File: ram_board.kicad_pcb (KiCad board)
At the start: 2 copper layers, 28.6 x 73 mm, 6 parts, among them J1 Conn_02x20_Odd_Even, J2 Conn_02x05_Odd_Even, U1 IS61LV5128AL-10TLI, U2 SST39VF040-70-4C-NHE

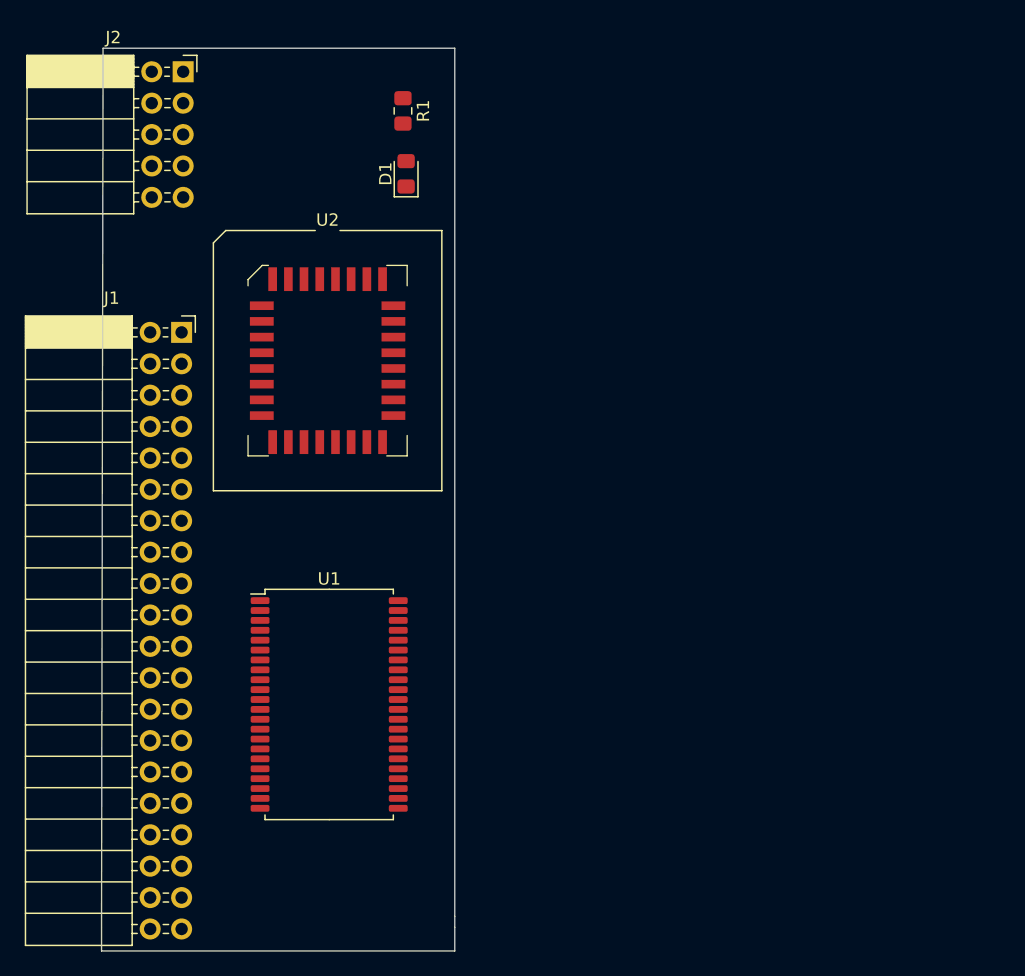
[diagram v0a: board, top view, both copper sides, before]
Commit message: Wiring up
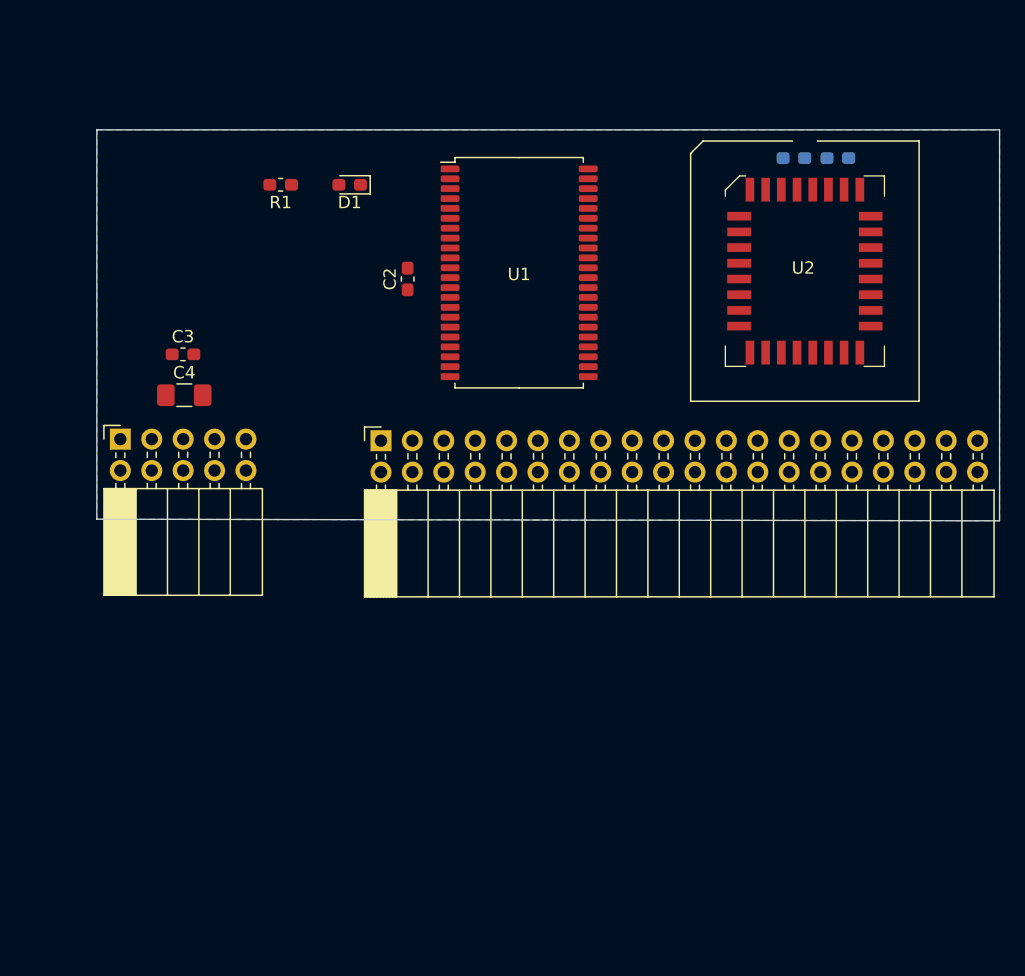
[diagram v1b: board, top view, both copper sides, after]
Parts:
- added C1: 100nF, Capacitor_SMD:C_0603_1608Metric_Pad1.05x0.95mm_HandSolder, B.Cu at (173.5, 74.8)
- added C2: 100nF, Capacitor_SMD:C_0603_1608Metric_Pad1.05x0.95mm_HandSolder, F.Cu at (142.2, 84.6)
- added C3: 100nF, Capacitor_SMD:C_0603_1608Metric_Pad1.05x0.95mm_HandSolder, F.Cu at (124.1, 90.7)
- added C4: 100uF, Capacitor_SMD:C_1206_3216Metric_Pad1.42x1.75mm_HandSolder, F.Cu at (124.2, 94.0)
- added G***: LOGO, Logos:asian_tiger, F.Cu at (160.8, 85.5)
- added R2: 10K, Resistor_SMD:R_0603_1608Metric_Pad1.05x0.95mm_HandSolder, B.Cu at (177.0, 74.8)
- D1: footprint LED_SMD:LED_0805_2012Metric_Pad1.15x1.40mm_HandSolder -> LED_SMD:LED_0603_1608Metric_Pad1.05x0.95mm_HandSolder
- R1: footprint Resistor_SMD:R_0805_2012Metric_Pad1.15x1.40mm_HandSolder -> Resistor_SMD:R_0603_1608Metric_Pad1.05x0.95mm_HandSolder
- moved U2 39.3 mm to (174.4, 83.9)
- moved U1 38.2 mm to (151.3, 84.1)
- moved J2 30.1 mm to (119.0, 97.5), turned to 90 degrees
- moved J1 18.4 mm to (140.1, 97.7), turned to 90 degrees
- moved R1 11.6 mm to (132.0, 77.0), turned to 180 degrees
- moved D1 4.65 mm to (137.6, 77.0), turned to 180 degrees
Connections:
- J1 pad 1: (no net) -> /A0
- J1 pad 10: (no net) -> /A9
- J1 pad 11: (no net) -> /A10
- J1 pad 12: (no net) -> /A11
- J1 pad 13: (no net) -> /A12
- J1 pad 14: (no net) -> /A13
- J1 pad 15: (no net) -> /A14
- J1 pad 16: (no net) -> /A15
- J1 pad 17: (no net) -> /A16
- J1 pad 18: (no net) -> /A17
- J1 pad 19: (no net) -> /A18
- J1 pad 2: (no net) -> /A1
- J1 pad 21: (no net) -> /RAM_CE
- J1 pad 22: (no net) -> /D0
- J1 pad 23: (no net) -> /RAM_OE
- J1 pad 24: (no net) -> /D1
- J1 pad 25: (no net) -> /RAM_WE
- J1 pad 26: (no net) -> /D2
- J1 pad 28: (no net) -> /D3
- J1 pad 3: (no net) -> /A2
- J1 pad 32: (no net) -> GND
- J1 pad 33: (no net) -> GND
- J1 pad 34: (no net) -> /D4
- J1 pad 36: (no net) -> /D5
- J1 pad 38: (no net) -> /D6
- J1 pad 39: (no net) -> GND
- J1 pad 4: (no net) -> /A3
- J1 pad 40: (no net) -> /D7
- J1 pad 5: (no net) -> /A4
- J1 pad 6: (no net) -> /A5
- J1 pad 7: (no net) -> /A6
- J1 pad 8: (no net) -> /A7
- J1 pad 9: (no net) -> /A8
- J2 pad 10: (no net) -> GND
- J2 pad 3: (no net) -> +3V3
- J2 pad 4: (no net) -> +3V3
- J2 pad 7: (no net) -> GND
- J2 pad 8: (no net) -> GND
- J2 pad 9: (no net) -> GND
- R1 pad 2: (no net) -> +3V3
- U1 pad 10: (no net) -> /D1
- U1 pad 11: Net-(U1-Pad11) -> +3V3
- U1 pad 12: Net-(U1-Pad12) -> GND
- U1 pad 13: (no net) -> /D2
- U1 pad 14: (no net) -> /D3
- U1 pad 15: (no net) -> /RAM_WE
- U1 pad 16: (no net) -> /A5
- U1 pad 17: (no net) -> /A6
- U1 pad 18: (no net) -> /A7
- U1 pad 19: (no net) -> /A8
- U1 pad 20: (no net) -> /A9
- U1 pad 26: (no net) -> /A10
- U1 pad 27: (no net) -> /A11
- U1 pad 28: (no net) -> /A12
- U1 pad 29: (no net) -> /A13
- U1 pad 3: (no net) -> /A0
- U1 pad 30: (no net) -> /A14
- U1 pad 31: (no net) -> /D4
- U1 pad 32: (no net) -> /D5
- U1 pad 33: Net-(U1-Pad11) -> +3V3
- U1 pad 34: Net-(U1-Pad12) -> GND
- U1 pad 35: (no net) -> /D6
- U1 pad 36: (no net) -> /D7
- U1 pad 37: (no net) -> /RAM_OE
- U1 pad 38: (no net) -> /A15
- U1 pad 39: (no net) -> /A16
- U1 pad 4: (no net) -> /A1
- U1 pad 40: (no net) -> /A17
- U1 pad 41: (no net) -> /A18
- U1 pad 5: (no net) -> /A2
- U1 pad 6: (no net) -> /A3
- U1 pad 7: (no net) -> /A4
- U1 pad 8: (no net) -> /RAM_CE
- U1 pad 9: (no net) -> /D0
- U2 pad 1: (no net) -> /A18
- U2 pad 10: (no net) -> /A2
- U2 pad 11: (no net) -> /A1
- U2 pad 12: (no net) -> /A0
- U2 pad 13: (no net) -> /D0
- U2 pad 14: (no net) -> /D1
- U2 pad 15: (no net) -> /D2
- U2 pad 17: (no net) -> /D3
- U2 pad 18: (no net) -> /D4
- U2 pad 19: (no net) -> /D5
- U2 pad 2: (no net) -> /A16
- U2 pad 20: (no net) -> /D6
- U2 pad 21: (no net) -> /D7
- U2 pad 22: (no net) -> /RAM_CE
- U2 pad 23: (no net) -> /A10
- U2 pad 24: (no net) -> /RAM_OE
- U2 pad 25: (no net) -> /A11
- U2 pad 26: (no net) -> /A9
- U2 pad 27: (no net) -> /A8
- U2 pad 28: (no net) -> /A13
- U2 pad 29: (no net) -> /A14
- U2 pad 3: (no net) -> /A15
- U2 pad 30: (no net) -> /A17
- U2 pad 31: (no net) -> Net-(R2-Pad1)
- U2 pad 32: (no net) -> +3V3
- U2 pad 4: (no net) -> /A12
- U2 pad 5: (no net) -> /A7
- U2 pad 6: (no net) -> /A6
- U2 pad 7: (no net) -> /A5
- U2 pad 8: (no net) -> /A4
- U2 pad 9: (no net) -> /A3
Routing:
- added copper zone on B.Cu, net GND
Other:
- board size 28.6 x 73 mm -> 73 x 31.6 mm
- rule trace_min: 0.2 -> 0.1524
- rule via_min_drill: 0.3 -> 0.3302
- rule via_min_size: 0.4 -> 0.6858
